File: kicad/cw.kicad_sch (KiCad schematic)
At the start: 92 parts, among them J1 AUDIO, J2 KEY, Q1 NPN, Q10 NPN, Q11 NPN, Q2 NMOS, Q3 NPN, Q4 NPN, Q5 NPN, Q6 NPN, Q7 NPN, Q8 NPN, Q9 NPN, SW2 TX/RX, SW3 FREQ_SELECT, SW4 PWR, U1 Si5351A-B-GT, U2 LM2596T-ADJ, U3 PCF8574TS, U4 RC1602A

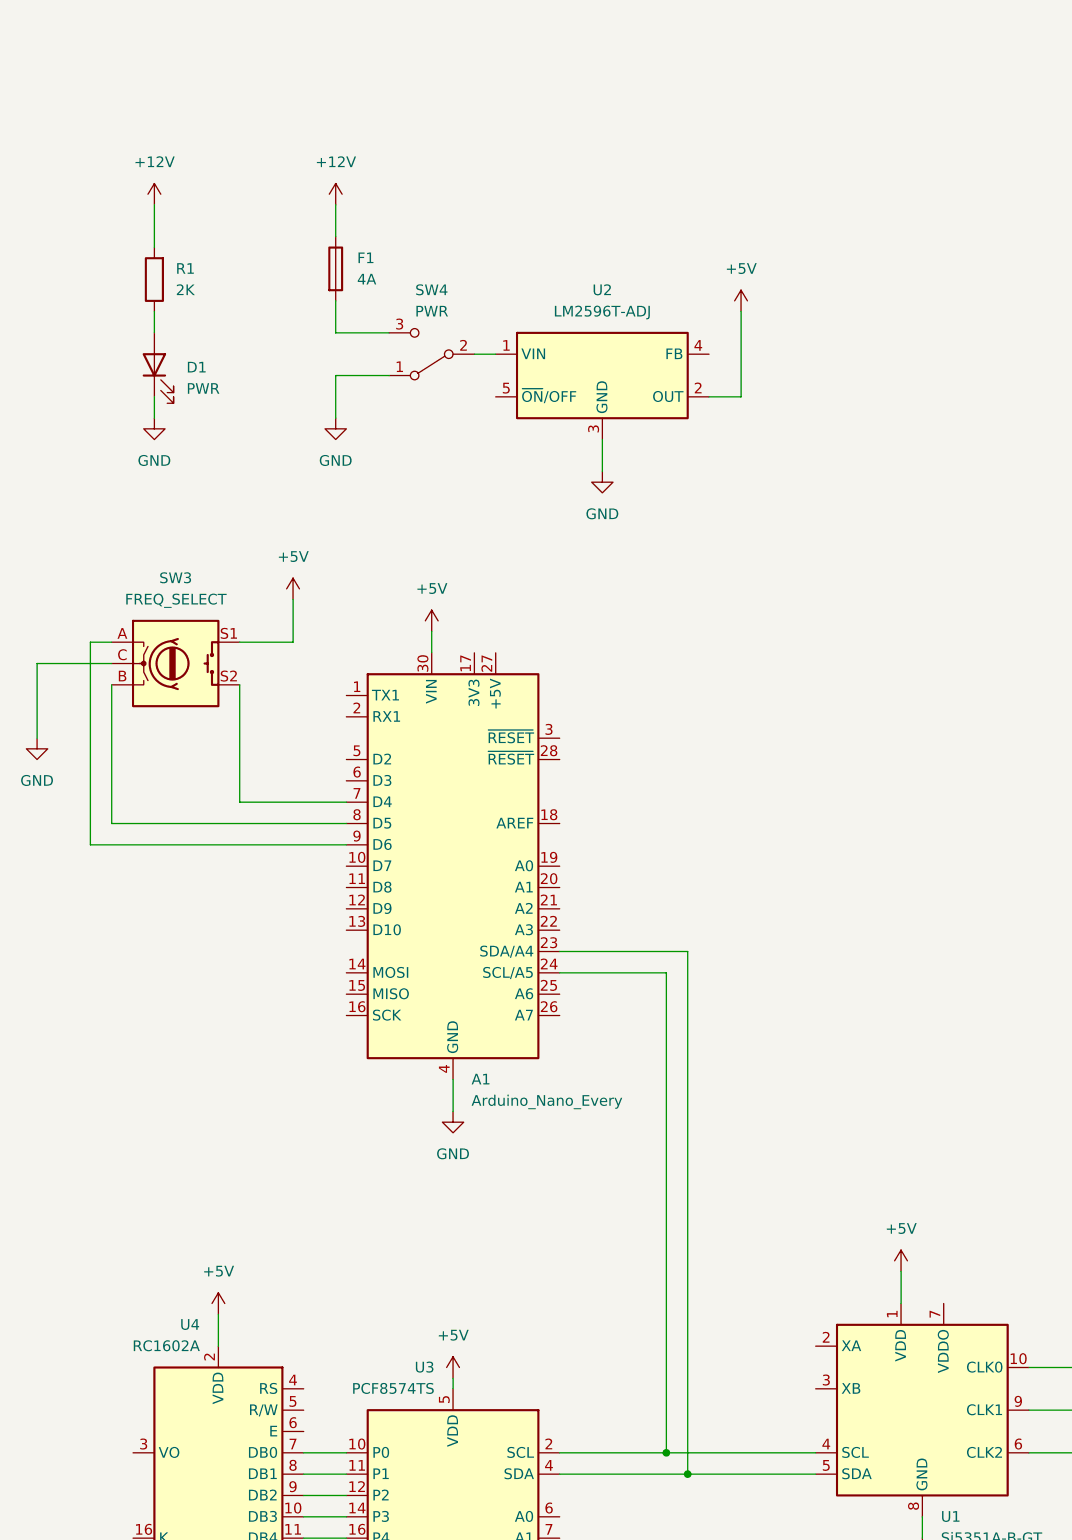
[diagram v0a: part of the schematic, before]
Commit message: Update cw.kicad_sch
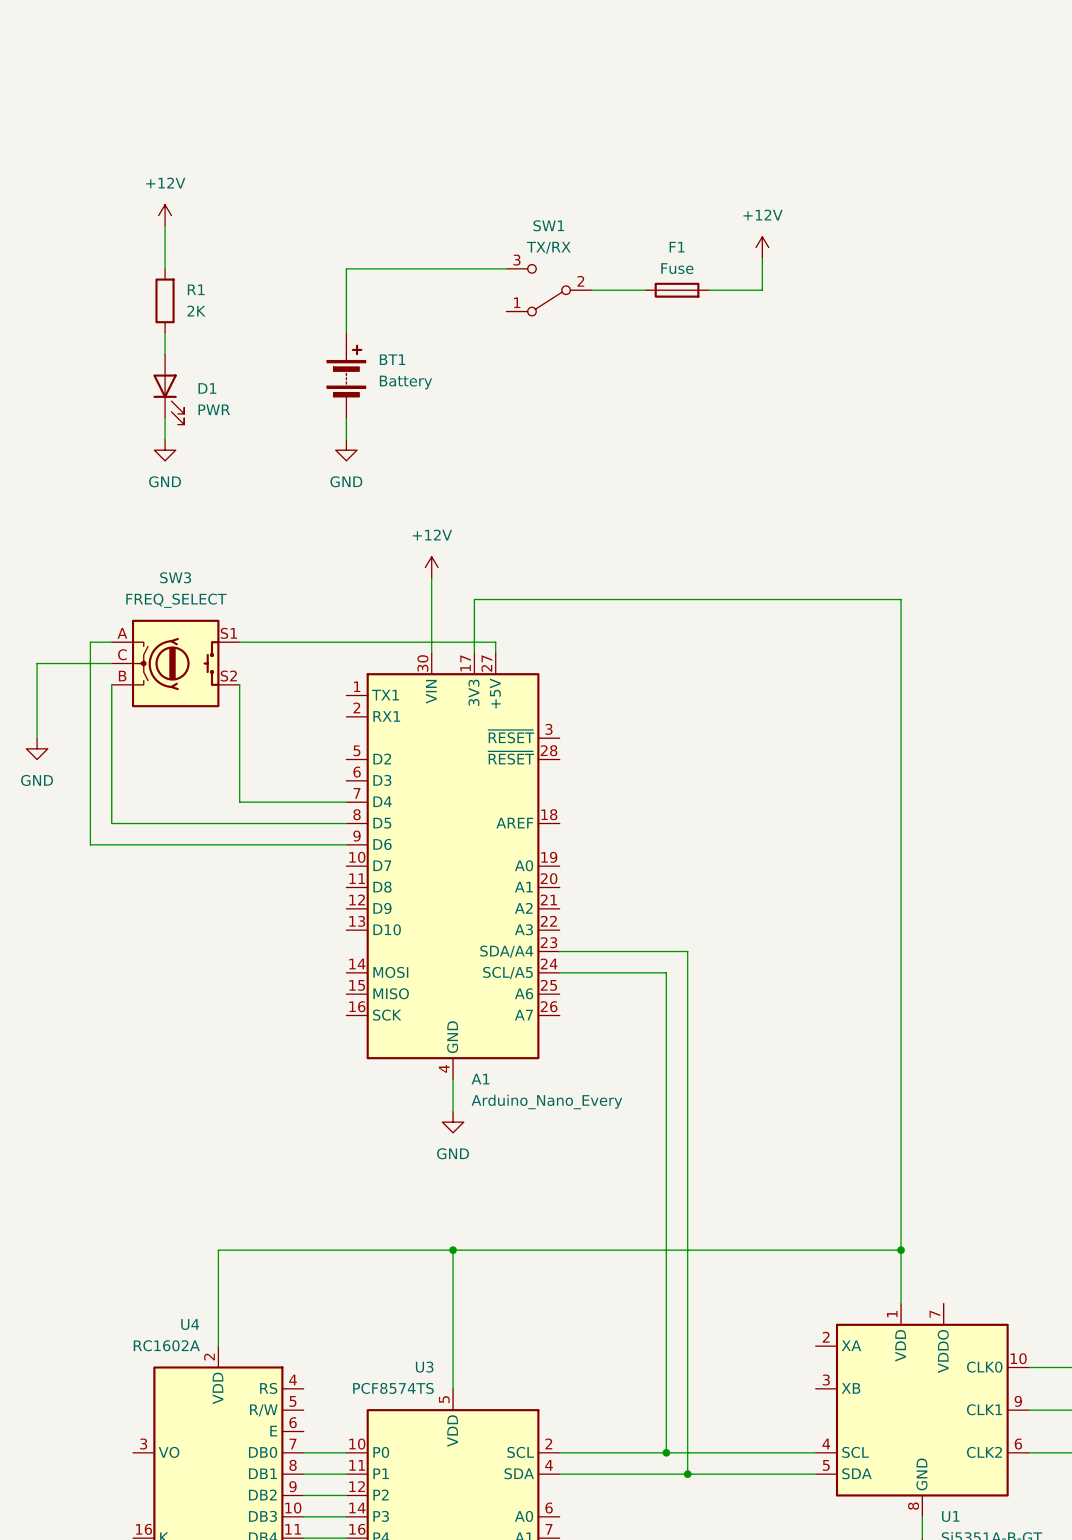
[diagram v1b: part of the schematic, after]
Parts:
- removed SW4: PWR, symbol Switch:SW_SPDT
- removed U2: LM2596T-ADJ, Package_TO_SOT_THT:TO-220-5_P3.4x3.7mm_StaggerOdd_Lead3.8mm_Vertical, symbol Regulator_Switching:LM2596T-ADJ
- added BT1: Battery, symbol Device:Battery
- added SW1: TX/RX, symbol Switch:SW_SPDT
- F1: value 4A -> Fuse
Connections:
- net +12V: now also A1.30 (VIN), F1.2; no longer F1.1
- net +5V: no longer A1.30 (VIN), SW3.S1, U1.1 (VDD), U3.5 (VDD), U4.2 (VDD)
- net GND: now also BT1.2 (-)
- net at A1.17 (3V3): now also U1.1 (VDD), U3.5 (VDD), U4.2 (VDD)
- net at A1.27 (+5V): now also SW3.S1
- new net: F1.1, SW1.2 (B)
- new net: BT1.1 (+), SW1.3 (C)
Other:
- moved on the sheet: D1, R1

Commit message: Update cw.kicad_sch
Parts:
- removed C13, C24, C25, C28, C29: C, symbol Device:C
- removed L21, L22, L24, L25, L9: L, symbol Device:L
- removed Q8, Q9: NPN, symbol Simulation_SPICE:NPN
- removed R9: R, symbol Device:R
- added Q12, Q13: NPN, symbol Simulation_SPICE:NPN
- added R12, R13, R14, R15, R16, R17, R18, R19, R20, R21, R22: R, symbol Device:R
- BT1: value Battery -> 12V
- F1: value Fuse -> 4A
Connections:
- net +12V: now also Q10.1 (C), Q11.1 (C), Q7.1 (C), R10.1, R7.1, Q12.1 (C), Q13.1 (C), R13.1, R14.1, R19.1
- net GND: now also R12.2, R15.2, R16.2, R17.2, R18.2, R20.2, R21.2, R22.2; no longer Q10.3 (E), Q11.3 (E), Q7.3 (E), R10.2, R7.2
- net at C12.2, Q5.2 (B), R4.1: now also Q7.2 (B), R7.2, R8.1
- net at C2.2, Q3.2 (B), R3.1: now also Q7.3 (E), R22.1
- net at L23.1: now also Q10.3 (E), R18.1; no longer Q7.1 (C)
- net at J2.S: now also Q11.3 (E), R12.1; no longer Q11.1 (C)
- net at Q11.2 (B), R11.1, U1.10 (CLK0): now also R13.2
- net at L11.1: now also Q13.3 (E), R21.1
- net at L16.2: now also Q12.3 (E), R16.1; no longer Q10.1 (C)
- new net: Q12.2 (B), R14.2, R15.1, U1.6 (CLK2)
- new net: Q10.2 (B), Q13.2 (B), R10.2, R17.1, R19.2, R20.1, U1.9 (CLK1)
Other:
- moved on the sheet: BT1, C18, C19, C22, C23, C26, D1, D4, F1, L13, L15, L16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

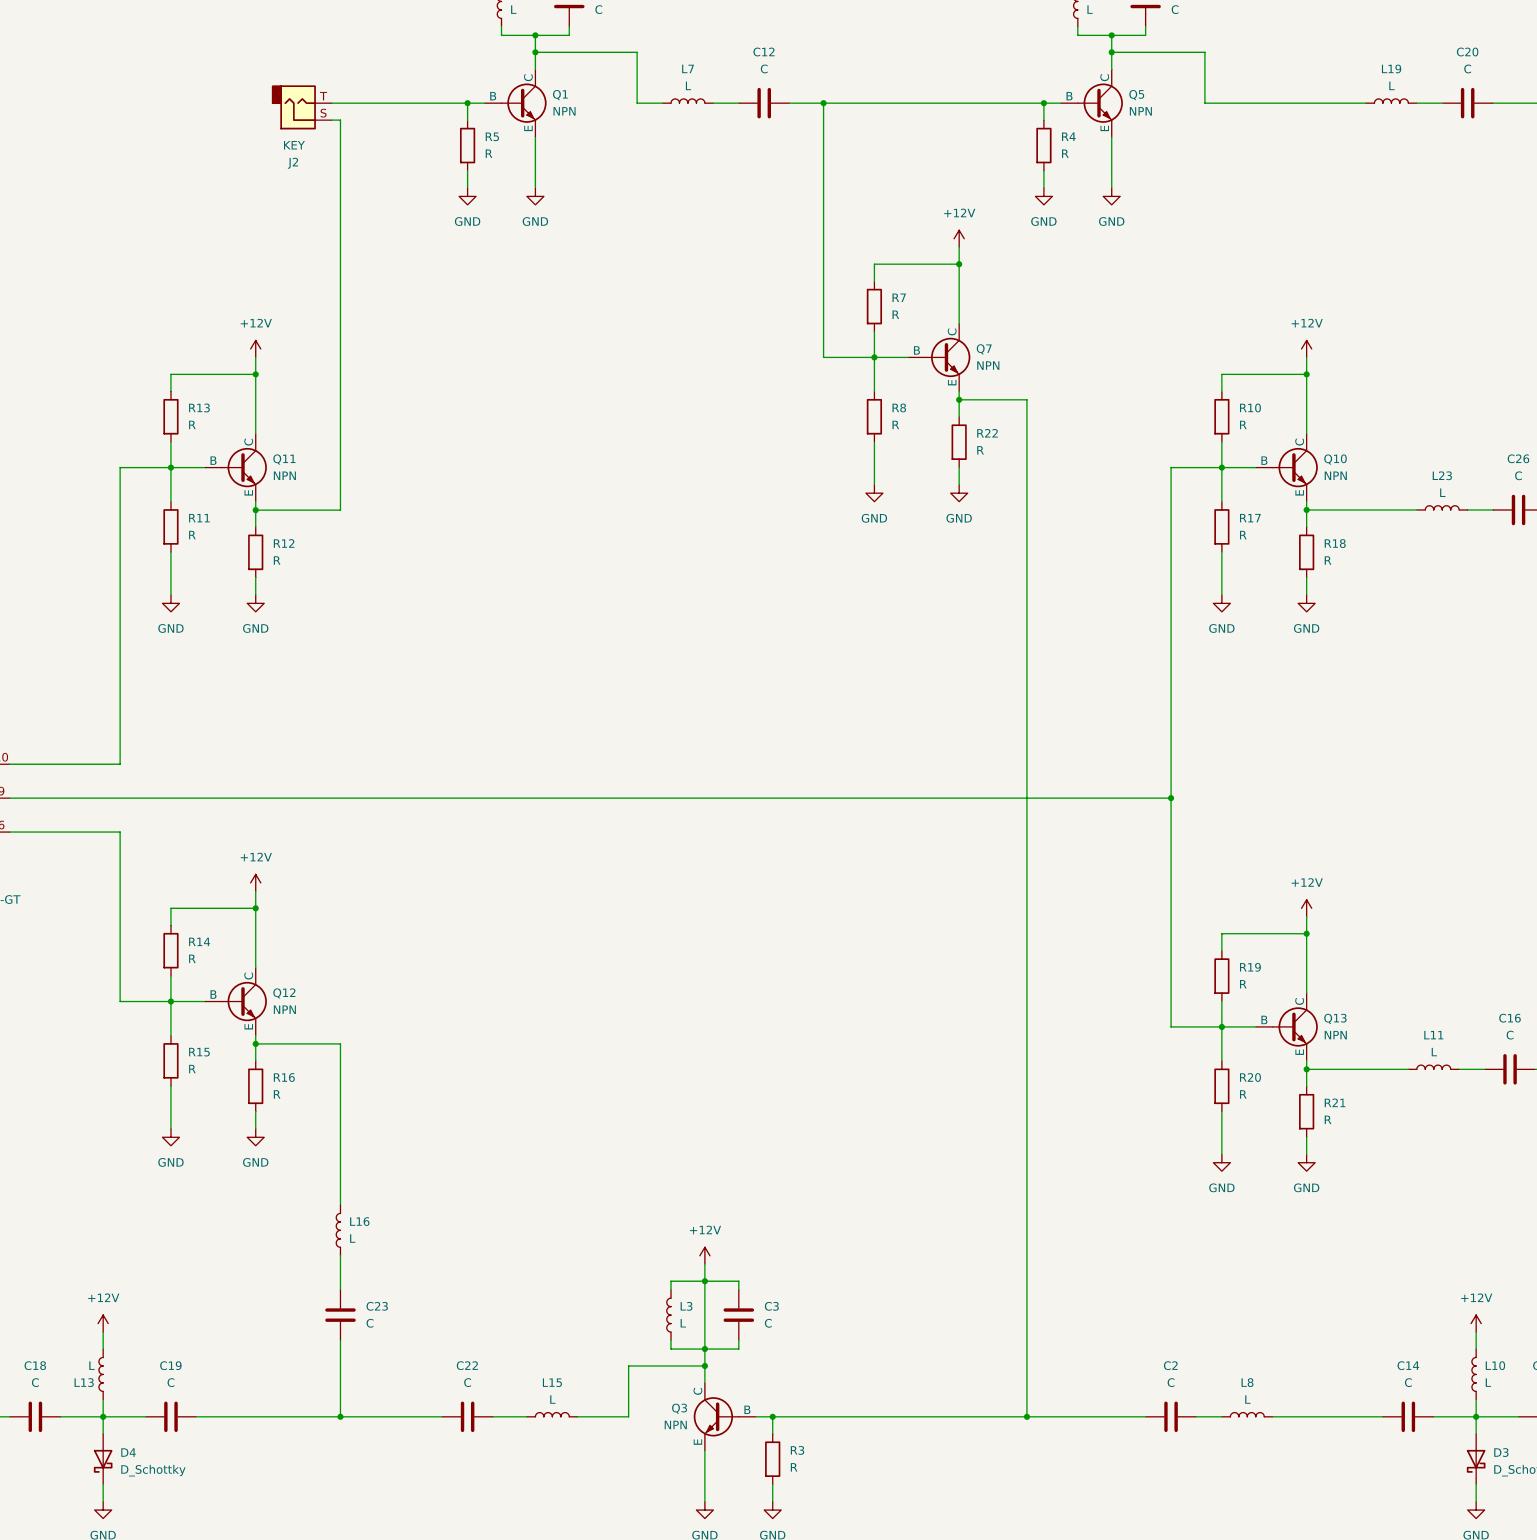
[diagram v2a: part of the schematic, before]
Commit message: Update cw.kicad_sch
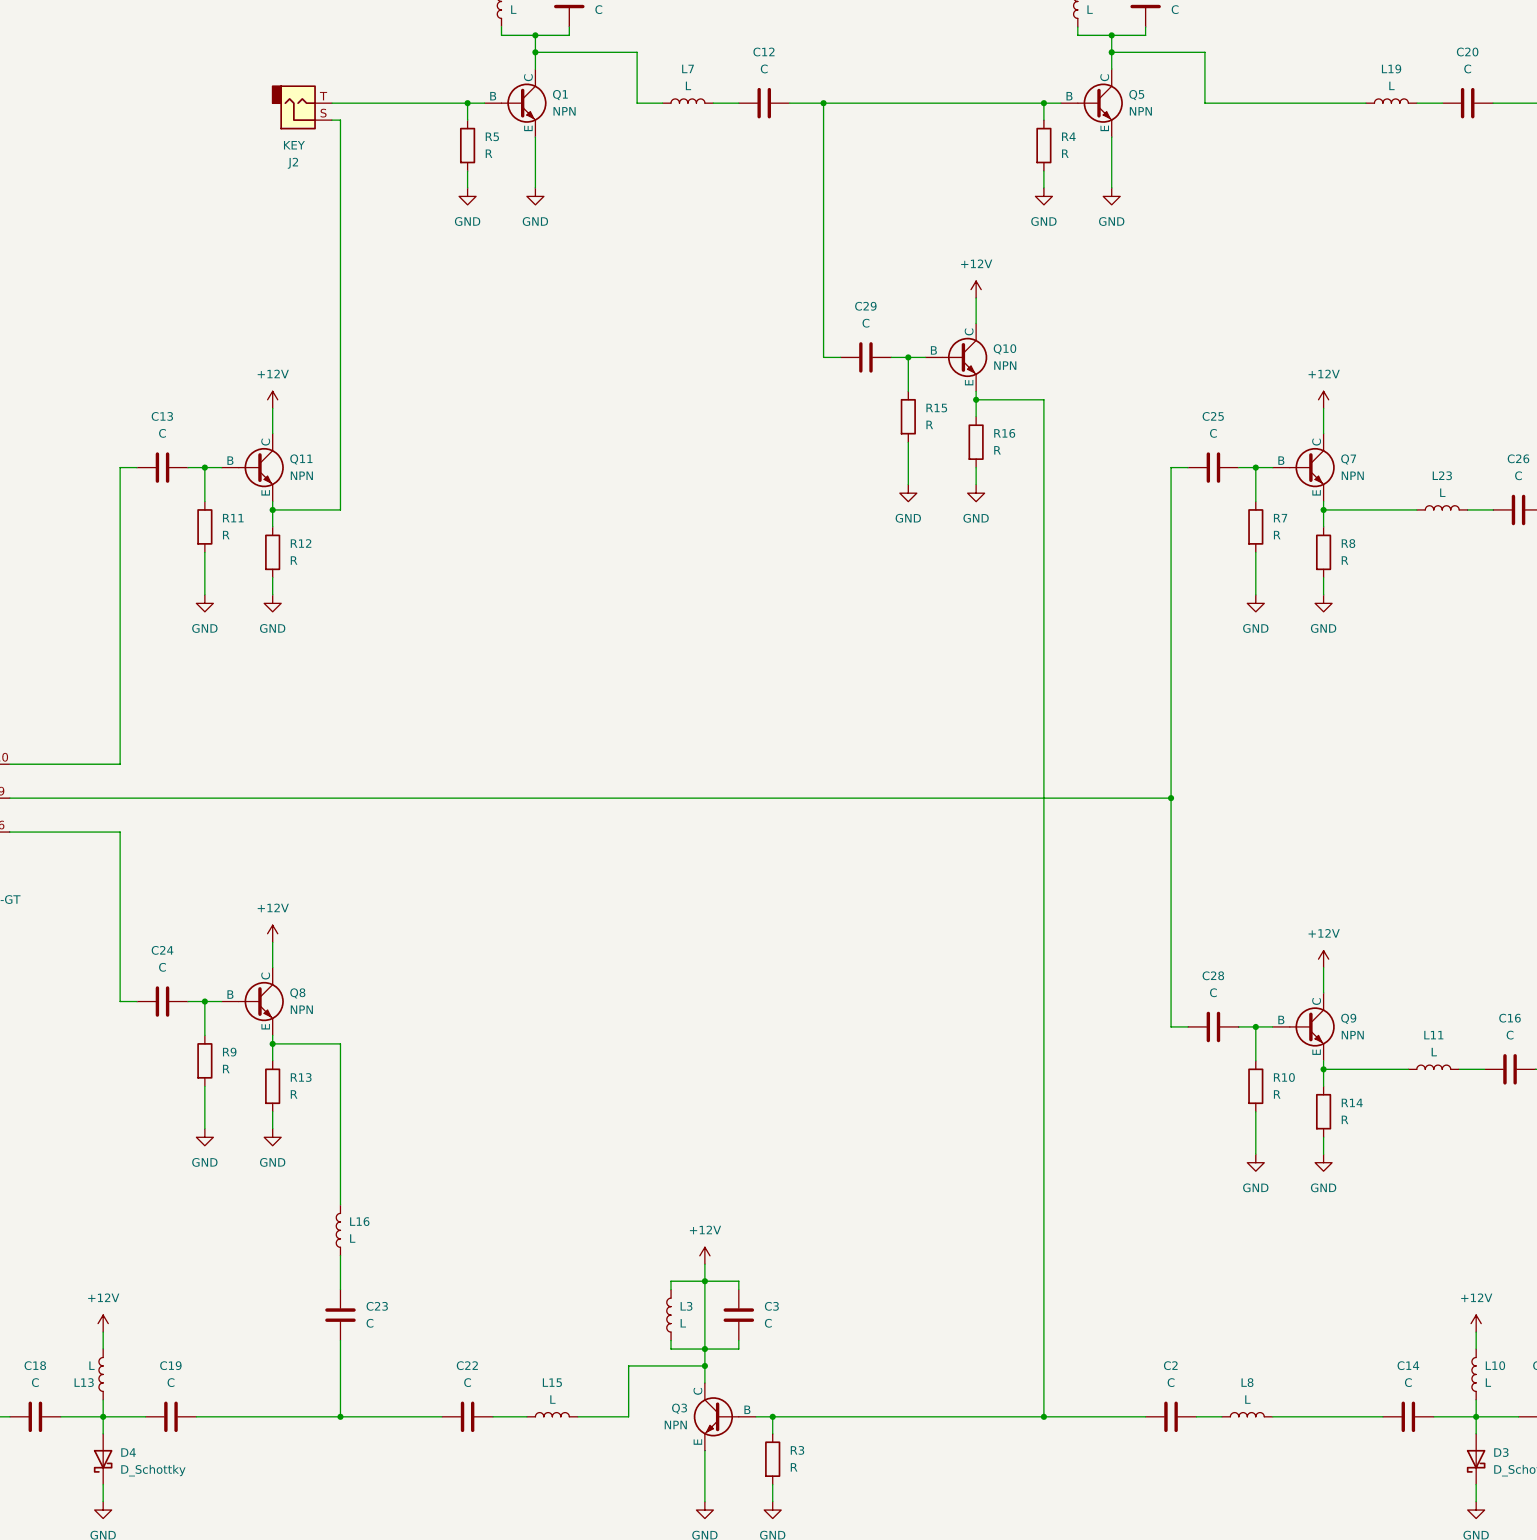
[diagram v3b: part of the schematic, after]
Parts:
- removed Q12, Q13: NPN, symbol Simulation_SPICE:NPN
- removed R17, R18, R19, R20, R21, R22: R, symbol Device:R
- added C13, C24, C25, C28, C29: C, symbol Device:C
- added Q8, Q9: NPN, symbol Simulation_SPICE:NPN
- added R9: R, symbol Device:R
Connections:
- net +12V: now also Q8.1 (C), Q9.1 (C); no longer R10.1, R13.1, R14.1, R7.1
- net GND: now also R10.2, R13.2, R14.2, R7.2, R9.2
- net at C12.2, Q5.2 (B), R4.1: now also C29.1; no longer Q7.2 (B), R7.2, R8.1
- net at C2.2, Q3.2 (B), R3.1: now also Q10.3 (E), R16.1; no longer Q7.3 (E)
- net at L23.1: now also Q7.3 (E), R8.1; no longer Q10.3 (E)
- net at L16.2: now also R13.1, Q8.3 (E); no longer R16.1
- net at Q11.2 (B), R11.1: now also C13.2; no longer R13.2, U1.10 (CLK0)
- net at L11.1: now also R14.1, Q9.3 (E)
- new net: C24.1, U1.6 (CLK2)
- new net: C24.2, Q8.2 (B), R9.1
- new net: C29.2, Q10.2 (B), R15.1
- new net: C13.1, U1.10 (CLK0)
- new net: C25.1, C28.1, U1.9 (CLK1)
- new net: C25.2, Q7.2 (B), R7.1
- new net: C28.2, Q9.2 (B), R10.1
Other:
- moved on the sheet: Q11, R11, R12
